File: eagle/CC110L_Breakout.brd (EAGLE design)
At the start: 20.9 x 30.9 mm, 28 parts

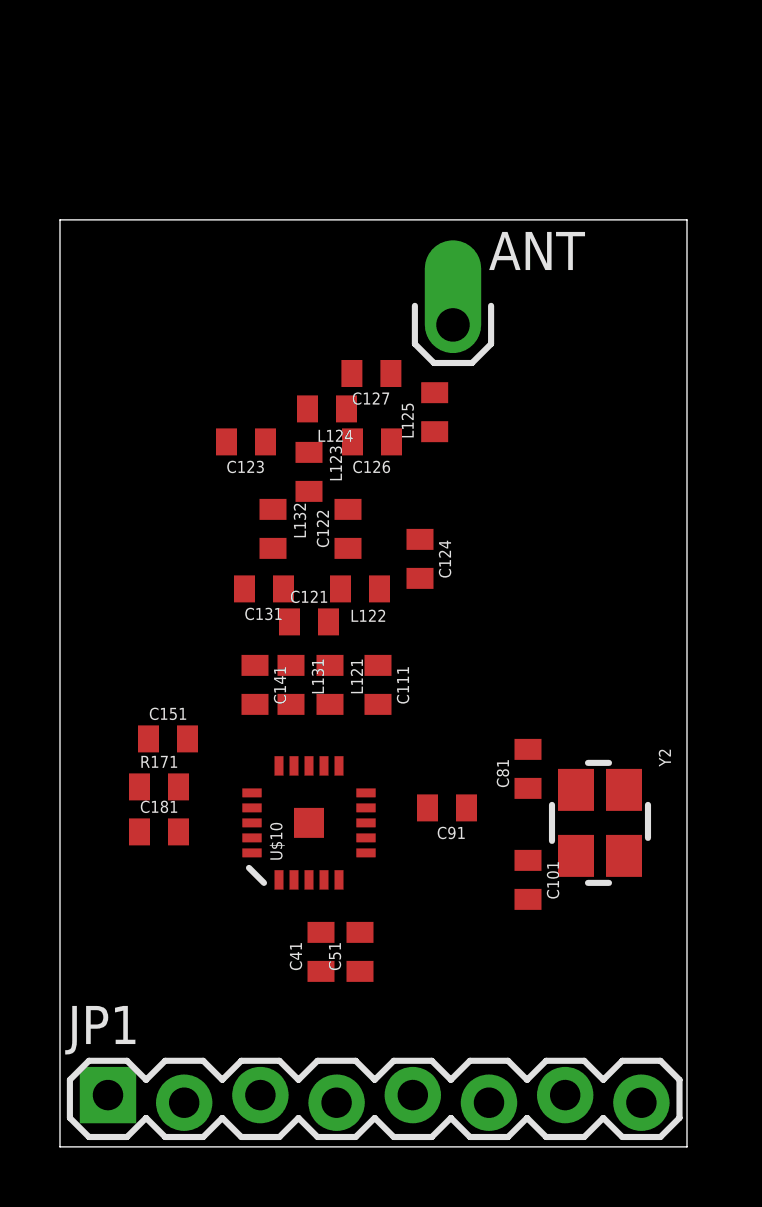
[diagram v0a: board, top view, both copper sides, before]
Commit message: almost completed board
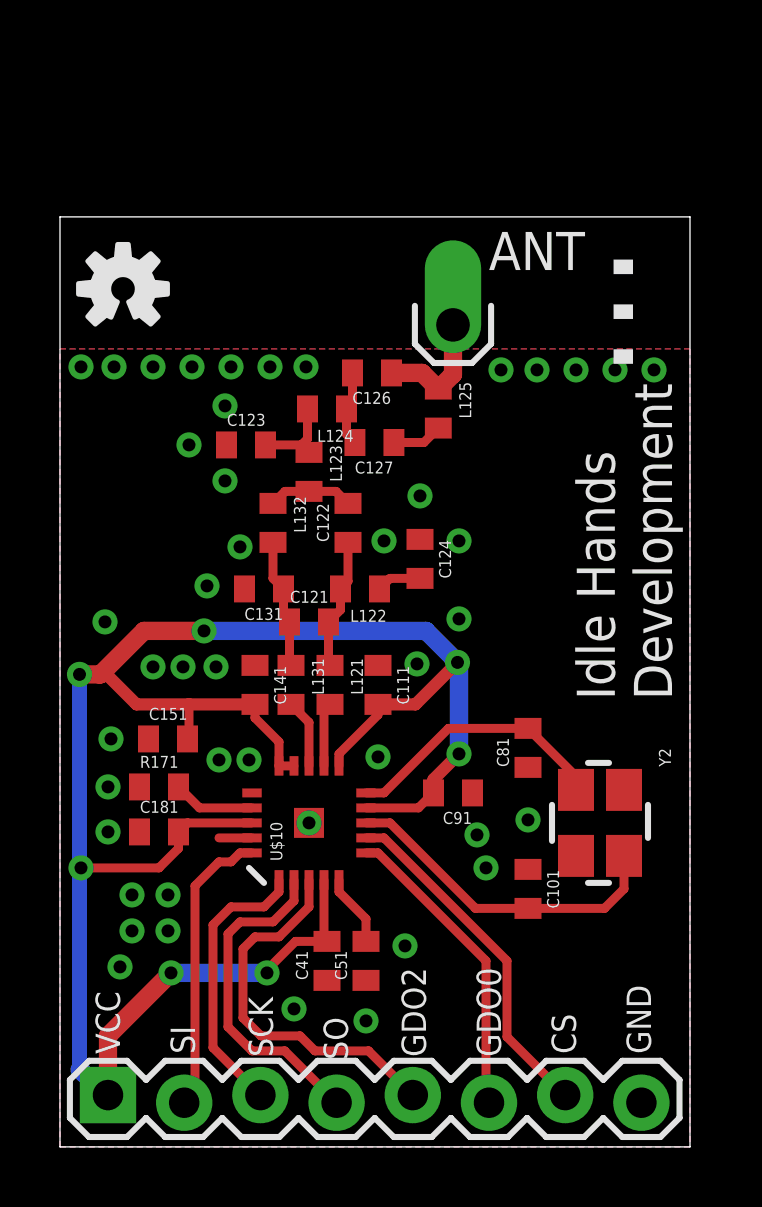
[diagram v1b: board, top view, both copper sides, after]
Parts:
- added LOGO1: OSHW-LOGOS, SparkFun-Aesthetics:OSHW-LOGO-S
- moved C127 2.30 mm to (10.5, 23.5)
- moved C126 2.30 mm to (10.4, 25.8)
- moved C81 0.70 mm to (15.6, 13.3)
- moved C91 0.54 mm to (13.1, 11.8)
- moved C41 0.36 mm to (8.90, 6.20)
- moved C51 0.36 mm to (10.2, 6.20)
- moved C101 0.30 mm to (15.6, 8.60)
- moved C122 0.20 mm to (9.60, 20.8)
- moved L132 0.20 mm to (7.10, 20.8)
- moved L125 0.17 mm to (12.6, 24.6), turned to 270 degrees
- moved C123 0.10 mm to (6.20, 23.4), turned to 0 degrees
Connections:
- net GDO0: now also JP1.6; no longer JP1.7
- net GDO2: now also JP1.5; no longer JP1.6
- net MISO: now also JP1.4; no longer JP1.3
- net RF_CS: now also JP1.7; no longer JP1.5
- net SCK: now also JP1.3; no longer JP1.4
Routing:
- net VCC: track 0.00 -> 70.7 mm, vias 0 -> 7
- net GDO2: track 0.00 -> 12.7 mm
- net RF_CS: track 0.00 -> 11.7 mm
- net N$12: track 0.00 -> 11.4 mm
- net MISO: track 0.00 -> 11.1 mm
- net GDO0: track 0.00 -> 10.3 mm
- net MOSI: track 0.00 -> 9.73 mm
- net SCK: track 0.00 -> 9.38 mm
- net N$13: track 0.00 -> 9.00 mm
- net N$5: track 0.00 -> 4.39 mm
- net N$2: track 0.00 -> 4.35 mm
- net N$11: track 0.00 -> 4.13 mm
- net N$8: track 0.00 -> 2.84 mm
- net N$7: track 0.00 -> 2.83 mm
- net N$16: track 0.00 -> 2.74 mm
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- added copper zone on layer 1, net GND
- added copper zone on layer 16, net GND
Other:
- board size 20.9 x 30.9 mm -> 21 x 31 mm
- board text added: "..."
- board text added: "CS"
- board text added: "GDO0"
- board text added: "GDO2"
- board text added: "GND"
- board text added: "Idle Hands Development"
- board text added: "SCK"
- board text added: "SI"
- board text added: "SO"
- board text added: "VCC"
